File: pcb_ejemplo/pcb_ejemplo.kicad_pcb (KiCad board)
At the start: 2 copper layers, 20.8 x 20.3 mm, 5 parts, among them J1 UPDI, U1 Microcontroller_ATtiny412_SSFR

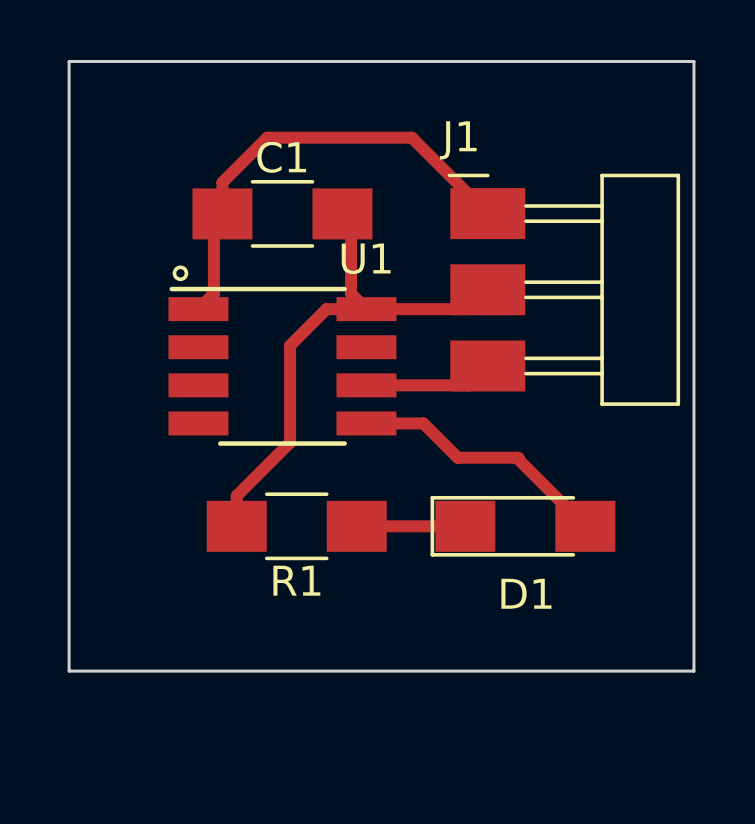
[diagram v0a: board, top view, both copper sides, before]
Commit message: update PCB
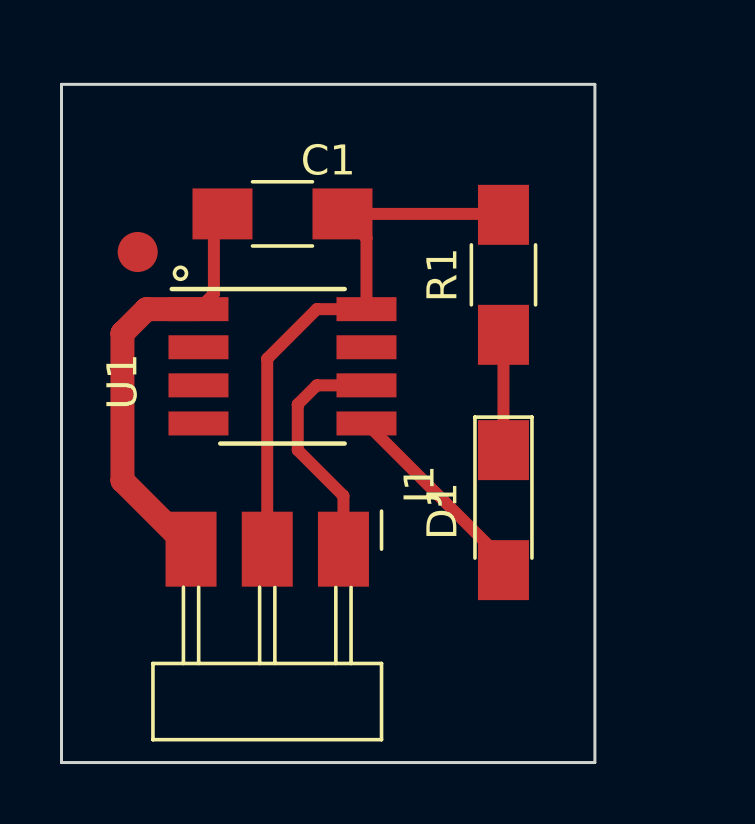
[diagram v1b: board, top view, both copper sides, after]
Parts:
- R1: value 1 k -> 499 Ohm
- moved J1 12.2 mm to (145.3, 109.0), turned to -90 degrees
- moved R1 10.9 mm to (150.6, 99.8), turned to 90 degrees
- moved D1 0.91 mm to (150.6, 107.7), turned to -90 degrees
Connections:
- J1 pad 1: PWR_5V -> UPDI
- J1 pad 3: UPDI -> PWR_5V
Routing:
- net UPDI: track 4.31 -> 8.01 mm
- net LED: track 8.78 -> 6.78 mm
- net PWR_GND: track 17.6 -> 19.2 mm
- net PWR_5V: track 15.1 -> 14.5 mm
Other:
- board size 20.8 x 20.3 mm -> 17.8 x 22.6 mm
